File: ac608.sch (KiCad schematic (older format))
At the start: 24 parts, among them J1 Conn_01x03, J2 Conn_01x03, J2 Jack-DC, J3 JTAG, P2 Conn_02x20_Odd_Even, P3 Conn_01x04, P4 Conn_01x02, P5 Conn_01x03, P6 Conn_01x03, P7 Conn_02x20_Odd_Even, P8 CAMERA, U1 LM1085-3.3

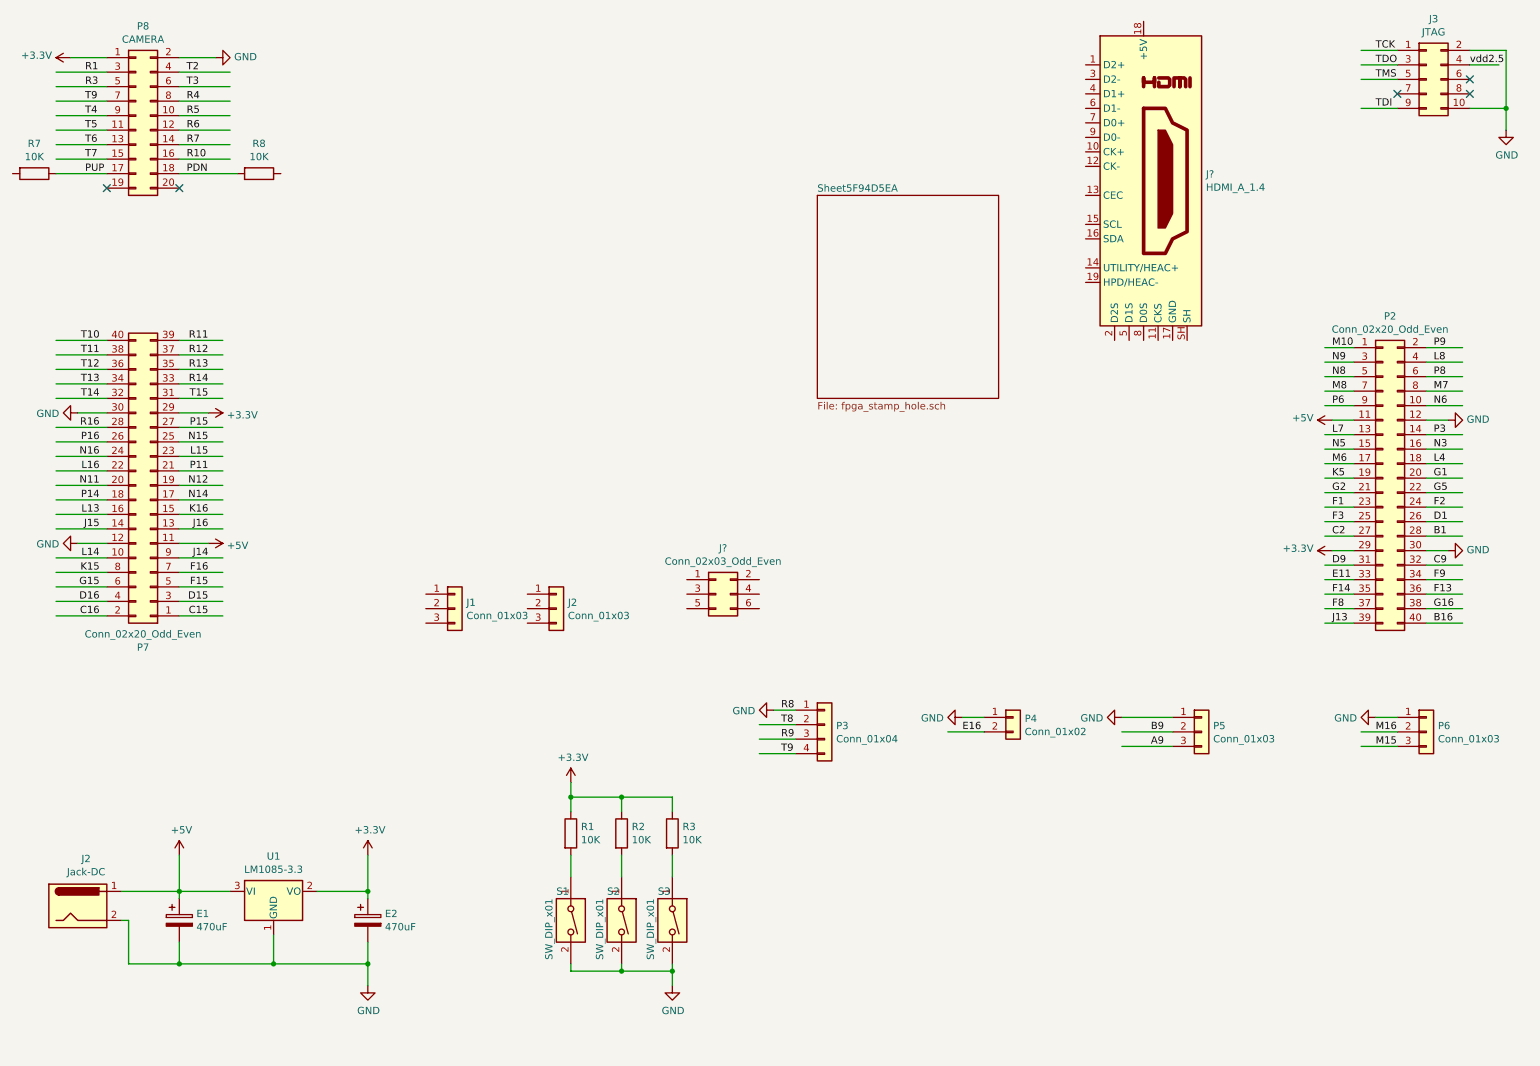
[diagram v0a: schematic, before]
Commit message: first commit
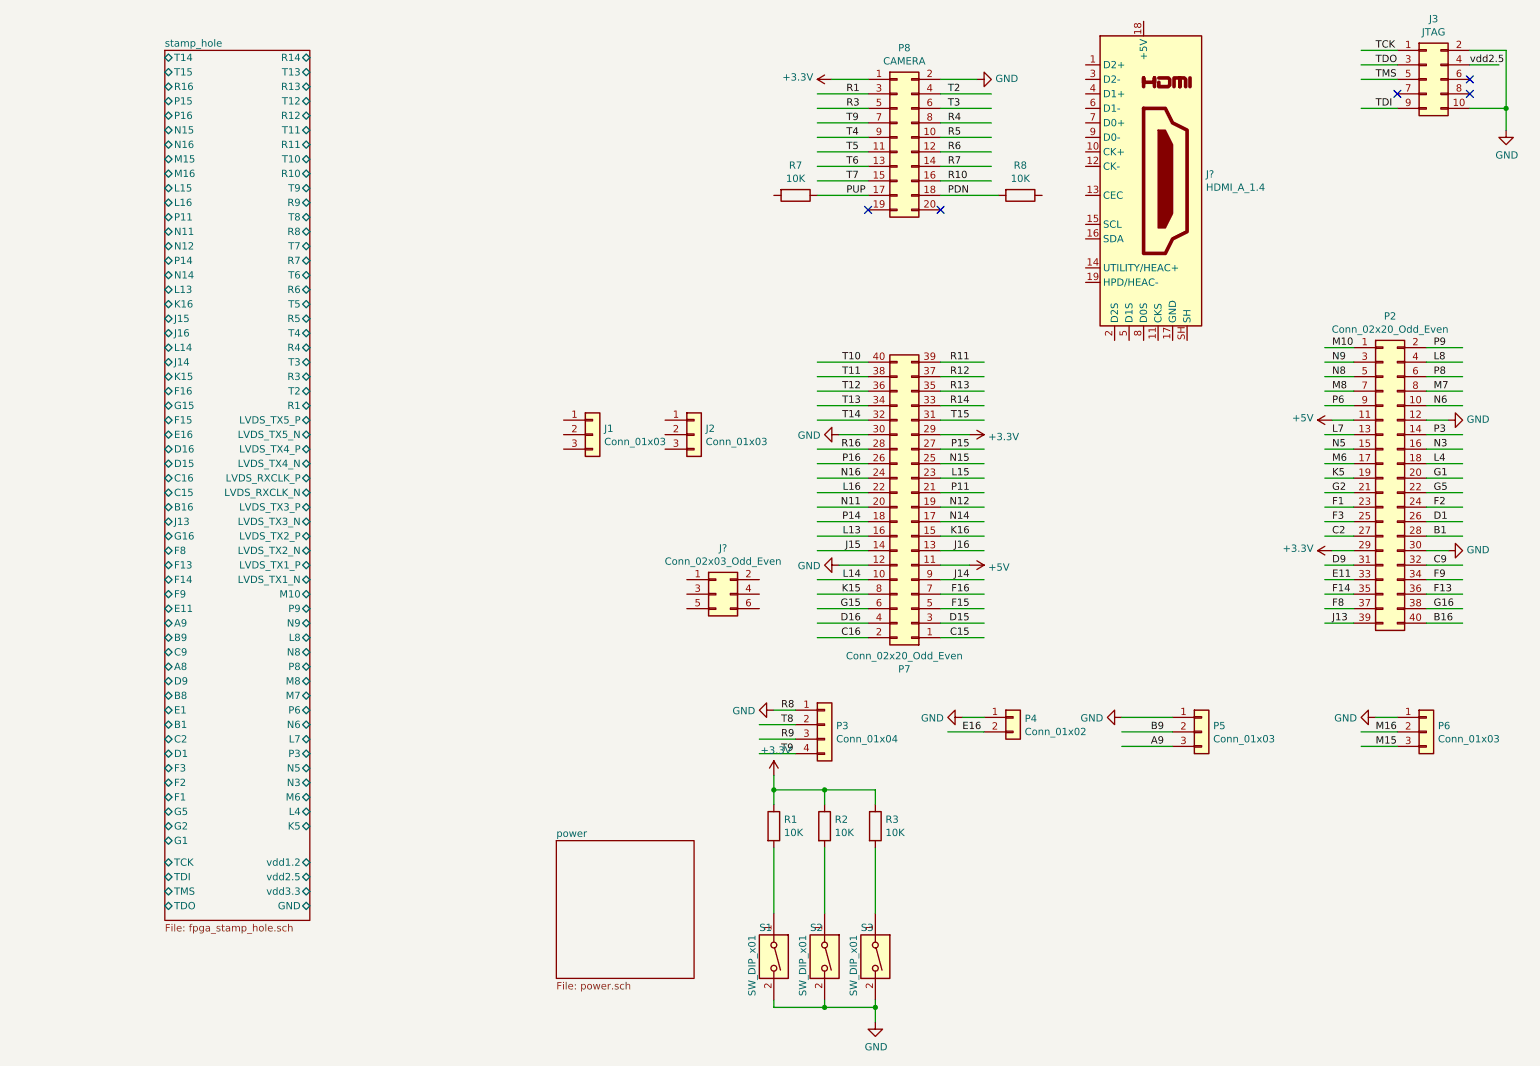
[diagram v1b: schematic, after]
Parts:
- removed E1, E2: 470uF, symbol Device:CP
- removed J2: Jack-DC, symbol Connector:Jack-DC
- removed U1: LM1085-3.3, symbol Regulator_Linear:LM1085-3.3
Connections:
- wire segments 150 -> 134
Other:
- moved on the sheet: J1, J2, P7, P8, R1, R2, R3, R7, R8, S1, S2, S3

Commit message: first commit
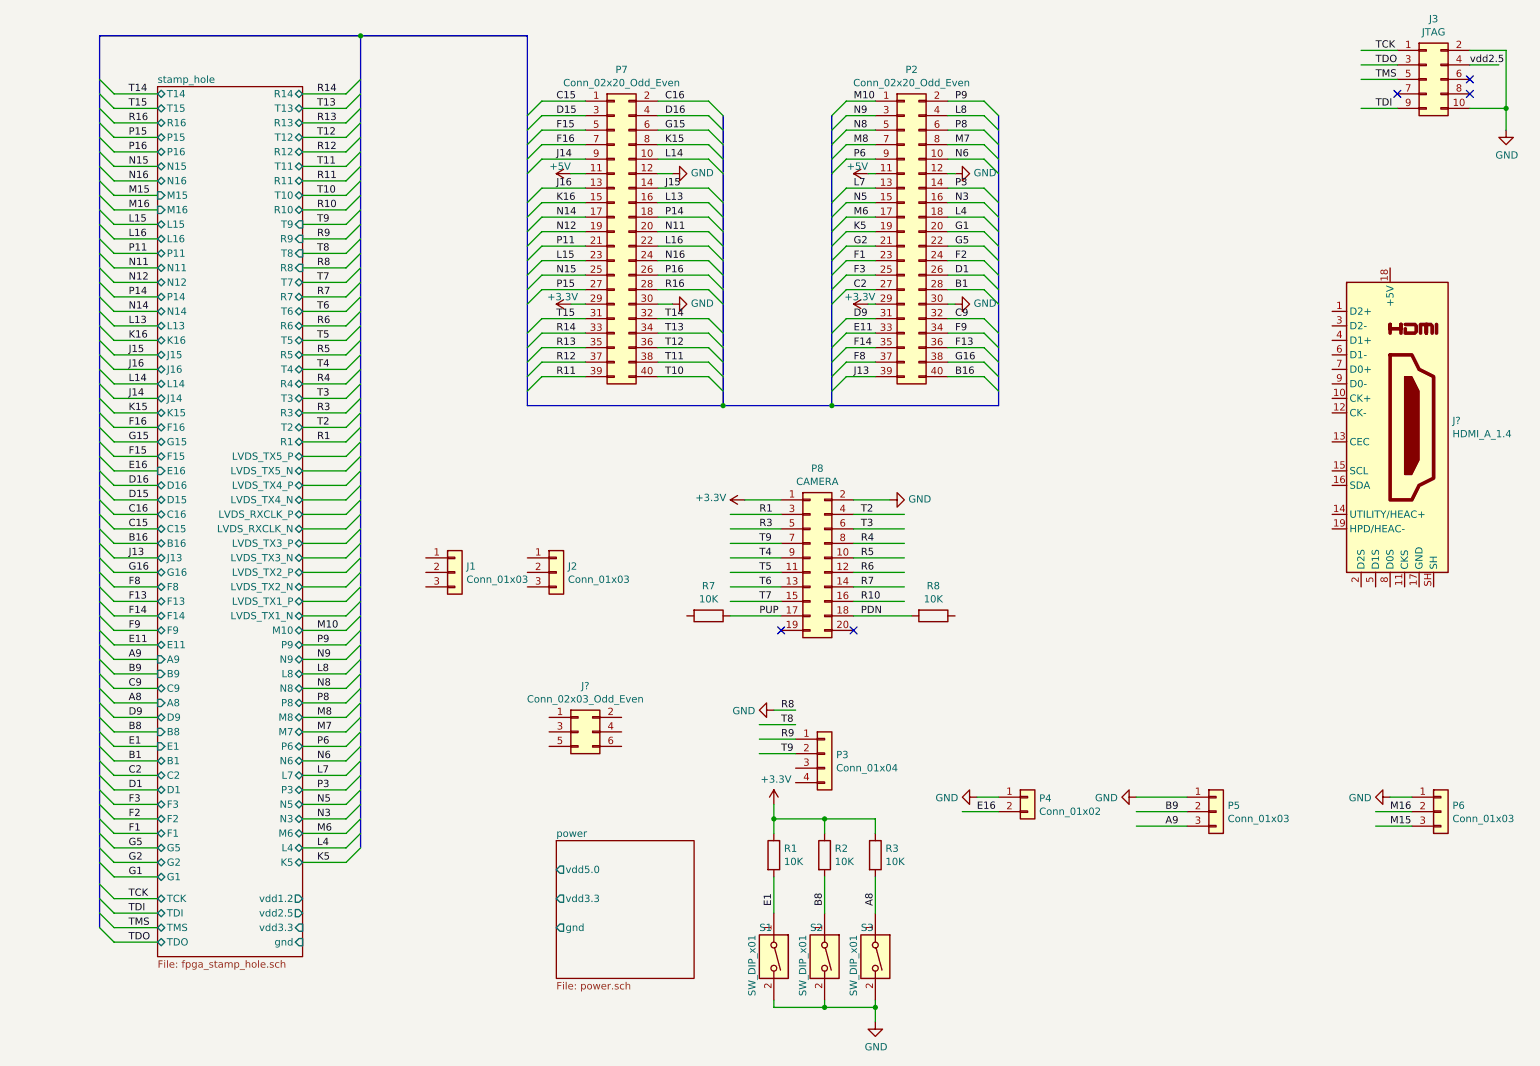
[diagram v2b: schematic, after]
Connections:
- net labels added: A8, B8, E1
- wire segments 134 -> 247
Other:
- moved on the sheet: J1, J2, J?, P2, P3, P4, P5, P6, P7, P8, R1, R2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

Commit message: first commit
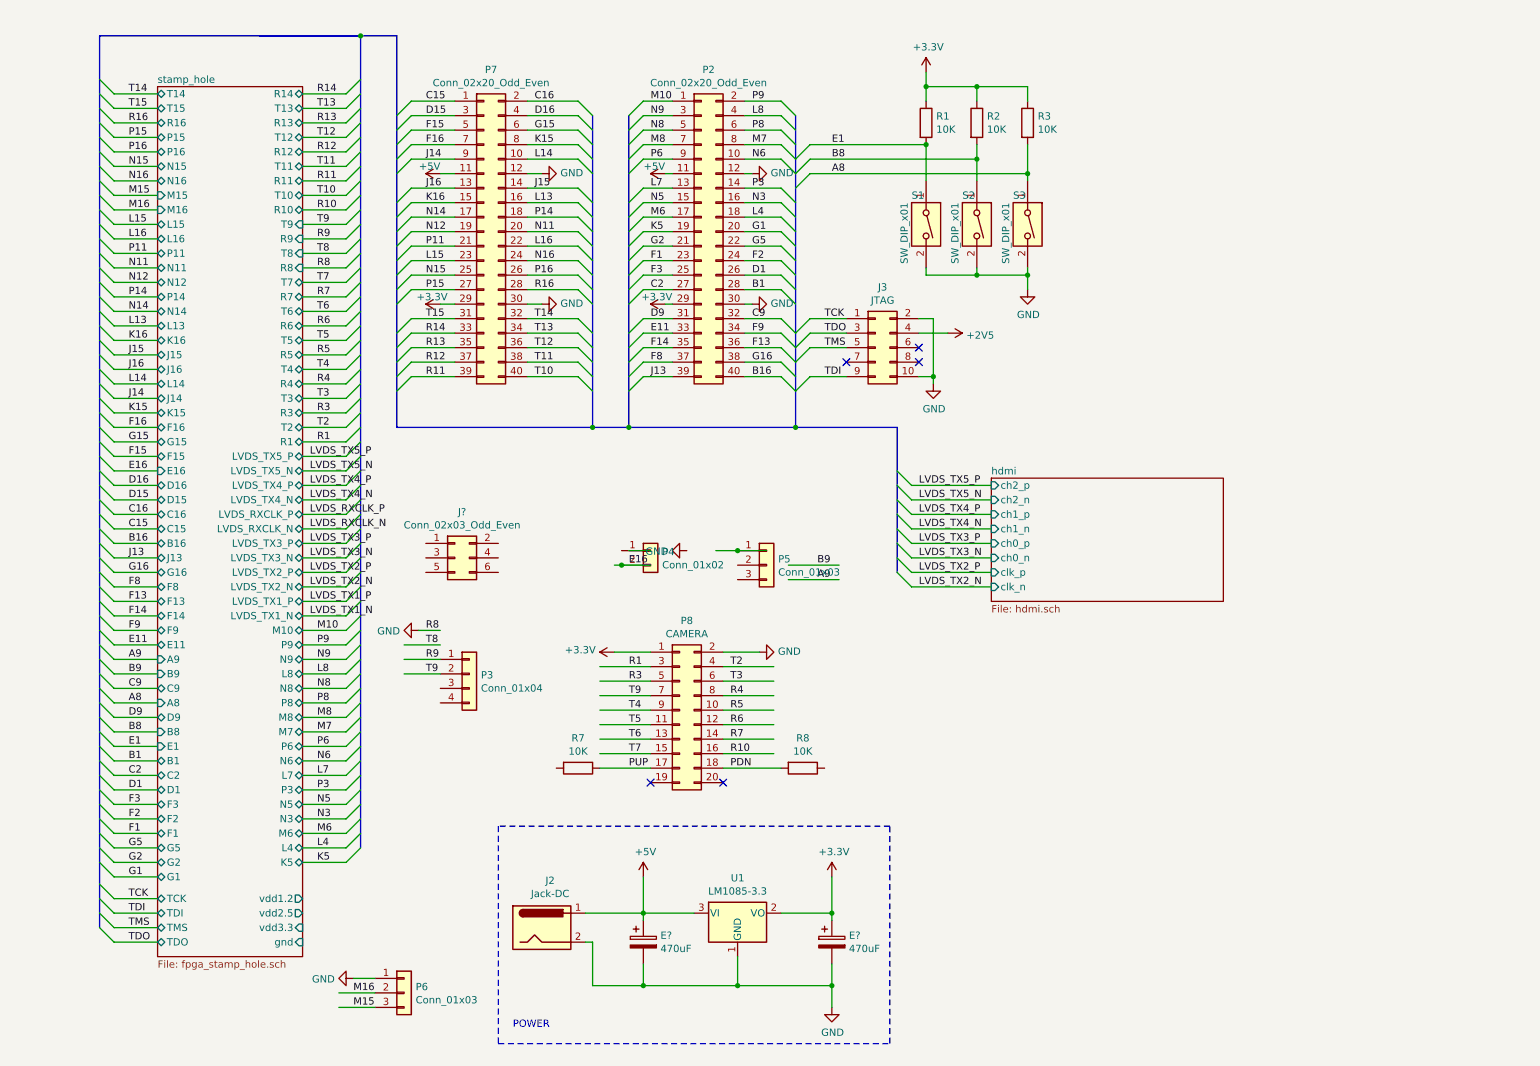
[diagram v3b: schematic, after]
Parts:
- removed J1, J2: Conn_01x03, symbol Connector_Generic:Conn_01x03
- removed J?: HDMI_A_1.4, symbol Connector:HDMI_A_1.4
- added E? (x2): 470uF, symbol Device:CP
- added J2: Jack-DC, symbol Connector:Jack-DC
- added U1: LM1085-3.3, symbol Regulator_Linear:LM1085-3.3
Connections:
- net labels added: +2V5, LVDS_RXCLK_N, LVDS_RXCLK_P, LVDS_TX1_N, LVDS_TX1_P, LVDS_TX2_N, LVDS_TX2_P, LVDS_TX3_N, LVDS_TX3_P, LVDS_TX4_N, LVDS_TX4_P, LVDS_TX5_N, LVDS_TX5_P
- net labels removed: vdd2.5
- wire segments 247 -> 278
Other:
- note added: "POWER"
- moved on the sheet: J3, J?, P2, P3, P4, P5, P6, P7, P8, R1, R2, R3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
